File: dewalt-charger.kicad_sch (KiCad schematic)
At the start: 1 part

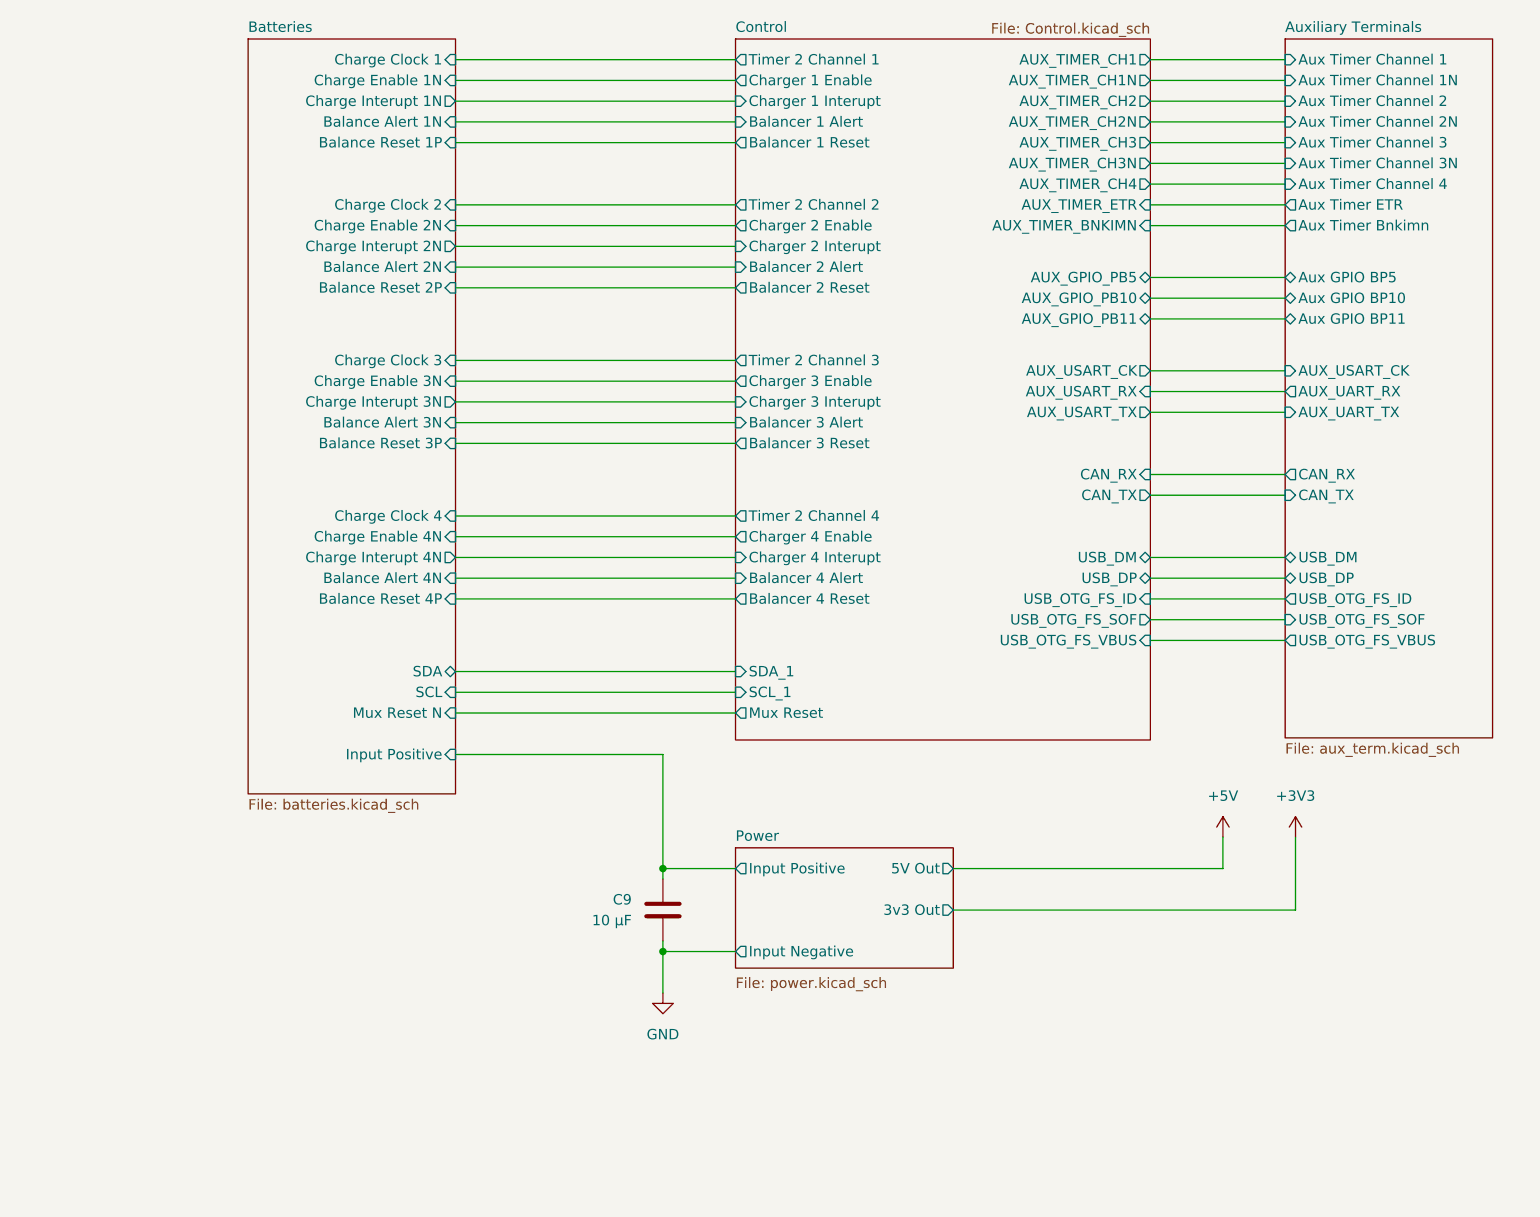
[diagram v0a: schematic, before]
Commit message: not adding this to source control months ago was one of the dumbest things i've ever done. and im not particularly risk-avers
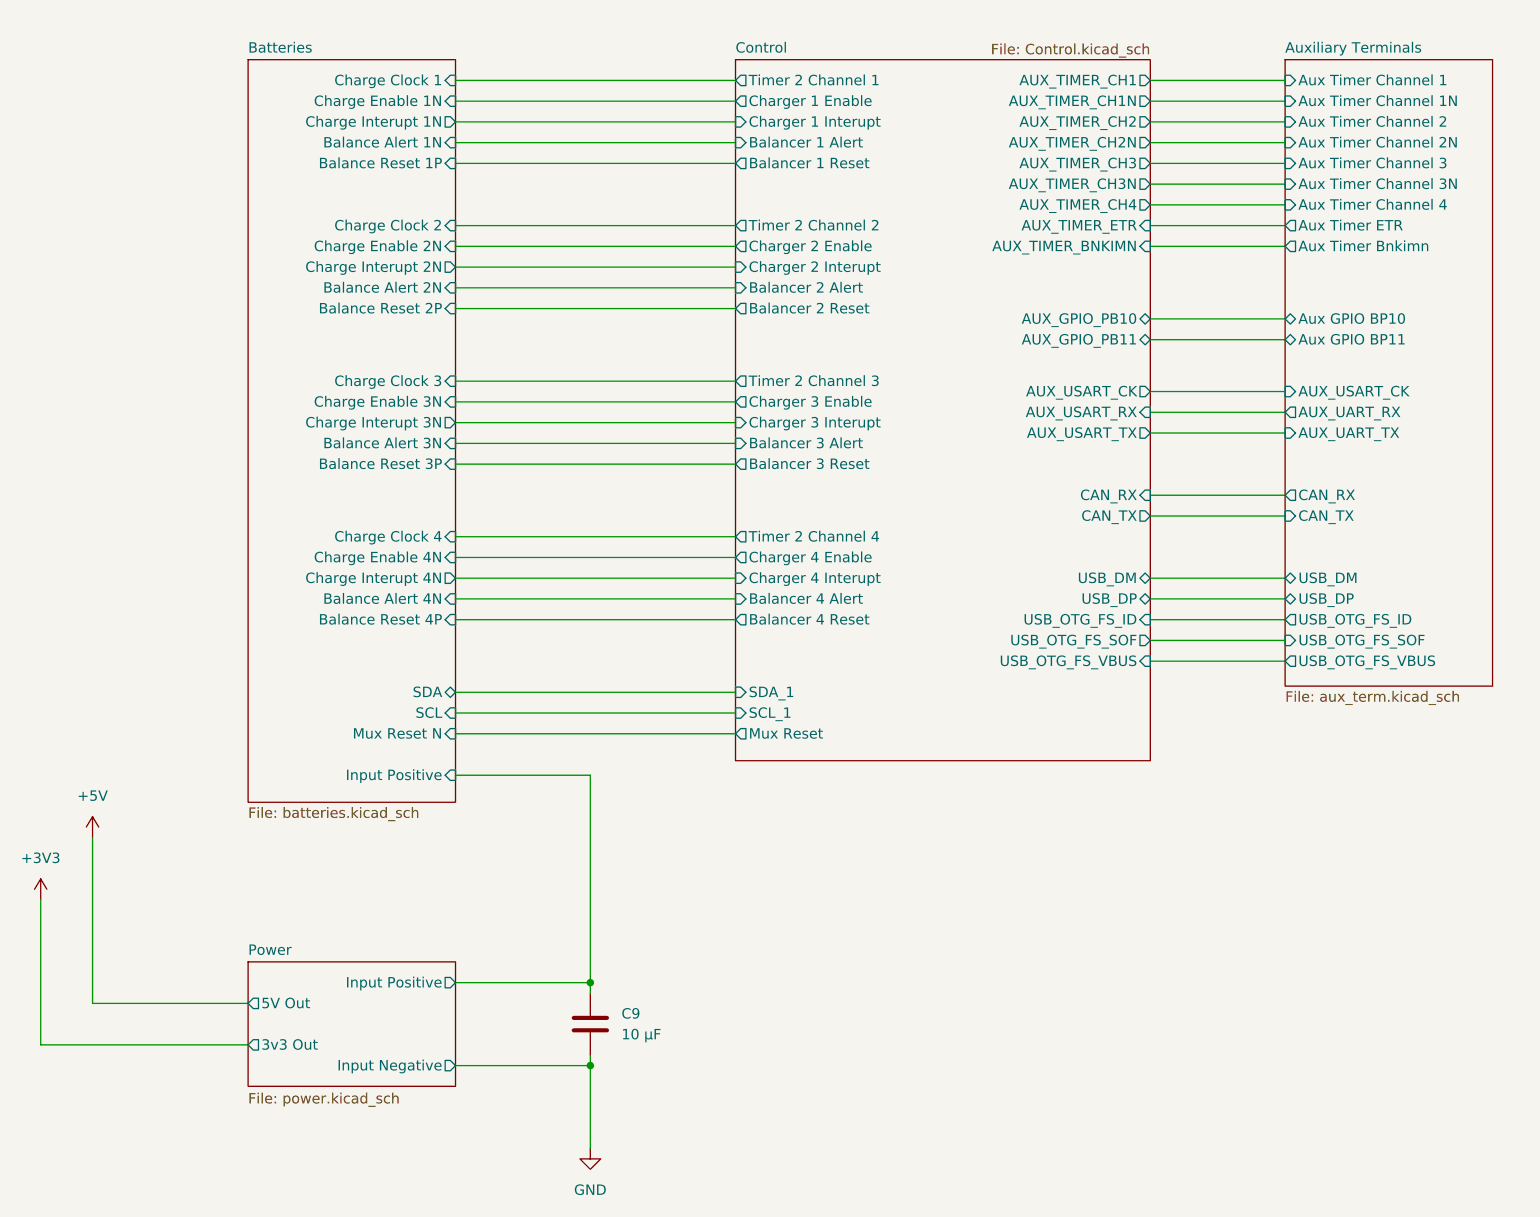
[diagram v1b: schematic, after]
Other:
- sheet Auxiliary Terminals ports: added none; removed Aux GPIO BP5
- sheet Control ports: added none; removed AUX_GPIO_PB5
- moved on the sheet: C9
